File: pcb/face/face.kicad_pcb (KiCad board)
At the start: 2 copper layers, 130 x 65 mm, 27 parts, among them J1 26 pin IDC, J2 Phoenix MSTB, U1 K155ID1, U2 K155ID1, U3 K155ID1, U4 K155ID1

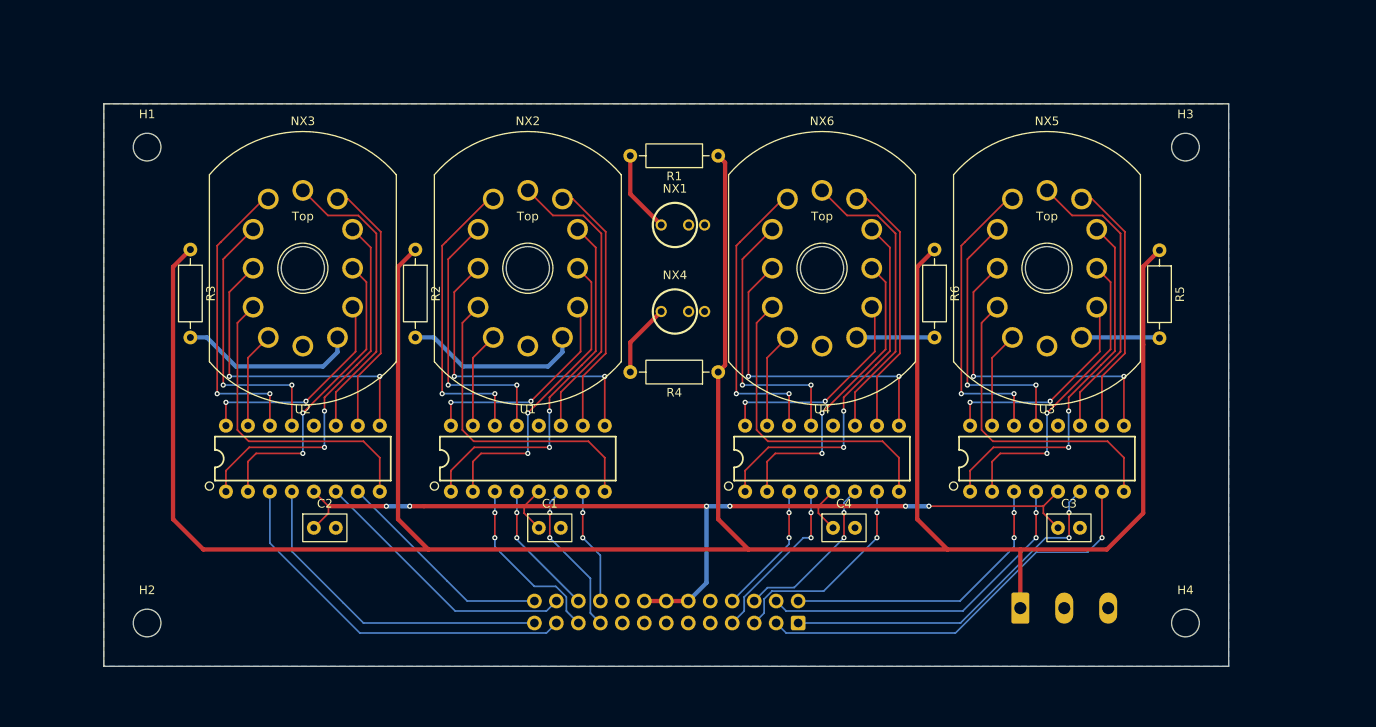
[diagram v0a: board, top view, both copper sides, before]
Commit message: Clock Face Rev C
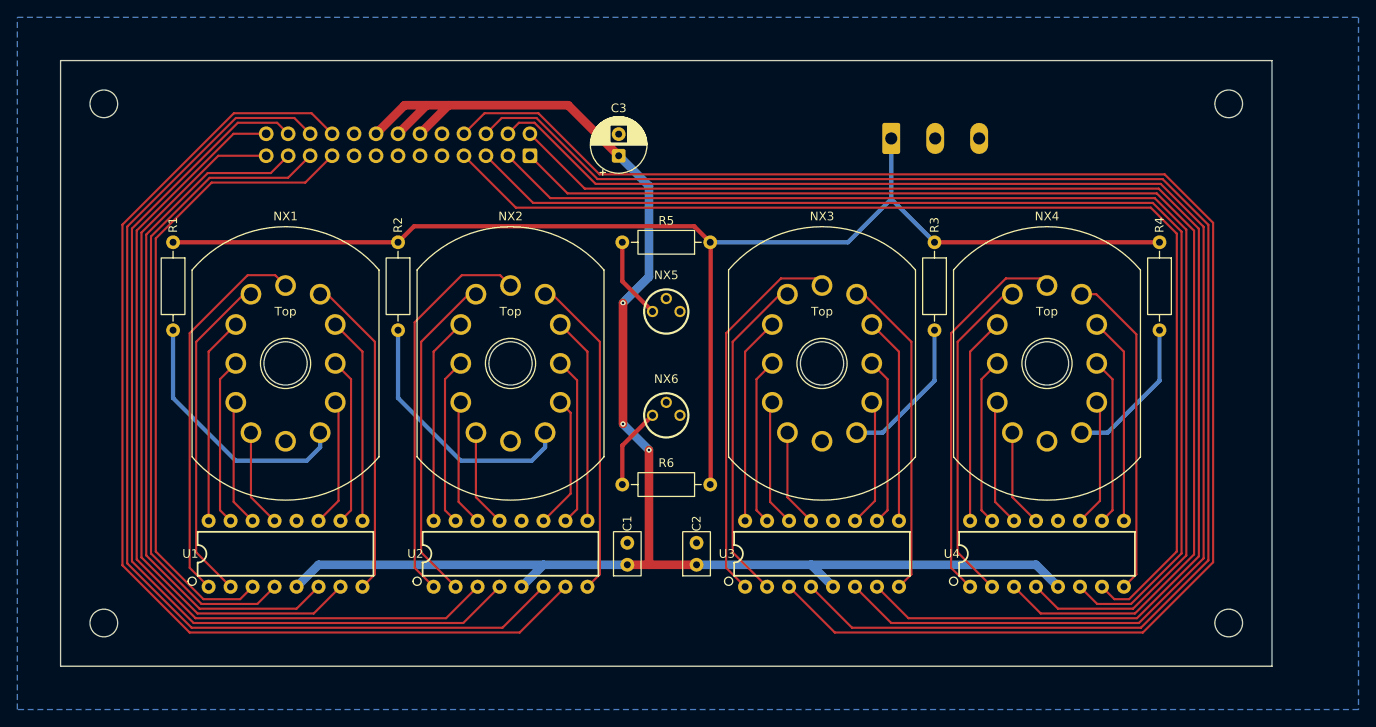
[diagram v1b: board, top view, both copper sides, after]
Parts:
- removed the C1 at (136.5, 109.0)
- C3: value 100nF -> 47uF; footprint 0_nixie_clock:C_Rect_L5.1mm_W3.2mm_P2.54mm_Goldmax -> 0_nixie_clock:CP_Radial_D6.3mm_P2.50mm
- moved C3 67.5 mm to (144.5, 66.0), turned to 90 degrees
- moved J1 62.3 mm to (134.2, 66.0)
- moved J2 56.3 mm to (176.0, 64.0)
- moved REF** 52.2 mm to (163.0, 64.0)
- moved C1 35.1 mm to (145.5, 112.0), turned to 90 degrees
- moved C2 17.3 mm to (153.5, 112.0), turned to 90 degrees
- moved R6 13.0 mm to (155.1, 104.0)
- moved NX6 12.0 mm to (150.0, 96.0)
- moved NX1 11.2 mm to (106.0, 90.0)
- moved NX2 11.2 mm to (132.0, 90.0)
- moved U1 11.2 mm to (106.0, 112.0)
- moved U2 11.2 mm to (132.0, 112.0)
- moved NX3 11.0 mm to (168.0, 90.0)
- moved NX4 11.0 mm to (194.0, 90.0)
- moved U3 11.0 mm to (168.0, 112.0)
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- renumbered C2 to C1, C4 to C2, NX3 to NX1, NX6 to NX3, NX5 to NX4, NX1 to NX5, NX4 to NX6, R3 to R1, R6 to R3, R5 to R4, R1 to R5, R4 to R6, U2 to U1, U1 to U2, U4 to U3, U3 to U4
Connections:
- J1 pad 1: M1_{B} -> M1_{A}
- J1 pad 19: H1_{B} -> H10_{A}
- J1 pad 2: M1_{A} -> M10_{C}
- J1 pad 21: H1_{A} -> H10_{D}
- J1 pad 22: H1_{D} -> H1_{B}
- J1 pad 23: H10_{A} -> H10_{B}
- J1 pad 24: H10_{B} -> H1_{D}
- J1 pad 25: H10_{D} -> H10_{C}
- J1 pad 26: H10_{C} -> H1_{A}
- J1 pad 3: M1_{C} -> M1_{D}
- J1 pad 4: M1_{D} -> M10_{B}
- J1 pad 5: M10_{C} -> M1_{B}
- J1 pad 6: M10_{B} -> M10_{D}
- J1 pad 7: M10_{D} -> M1_{C}
- NX1 pad 0: /NX1_{0} -> NX1_{0}
- NX1 pad 1: /NX1_{1} -> NX1_{1}
- NX1 pad 2: /NX1_{2} -> NX1_{2}
- NX1 pad 3: /NX1_{3} -> NX1_{3}
- NX1 pad 4: /NX1_{4} -> NX1_{4}
- NX1 pad 5: /NX1_{5} -> NX1_{5}
- NX1 pad 6: /NX1_{6} -> NX1_{6}
- NX1 pad 7: /NX1_{7} -> NX1_{7}
- NX1 pad 8: /NX1_{8} -> NX1_{8}
- NX1 pad 9: /NX1_{9} -> NX1_{9}
- NX2 pad 0: /NX2_{0} -> NX2_{0}
- NX2 pad 1: /NX2_{1} -> NX2_{1}
- NX2 pad 2: /NX2_{2} -> NX2_{2}
- NX2 pad 3: /NX2_{3} -> NX2_{3}
- NX2 pad 4: /NX2_{4} -> NX2_{4}
- NX2 pad 5: /NX2_{5} -> NX2_{5}
- NX2 pad 6: /NX2_{6} -> NX2_{6}
- NX2 pad 7: /NX2_{7} -> NX2_{7}
- NX2 pad 8: /NX2_{8} -> NX2_{8}
- NX2 pad 9: /NX2_{9} -> NX2_{9}
- NX3 pad 0: /NX3_{0} -> NX3_{0}
- NX3 pad 1: /NX3_{1} -> NX3_{1}
- NX3 pad 2: /NX3_{2} -> NX3_{2}
- NX3 pad 3: /NX3_{3} -> NX3_{3}
- NX3 pad 4: /NX3_{4} -> NX3_{4}
- NX3 pad 5: /NX3_{5} -> NX3_{5}
- NX3 pad 6: /NX3_{6} -> NX3_{6}
- NX3 pad 7: /NX3_{7} -> NX3_{7}
- NX3 pad 8: /NX3_{8} -> NX3_{8}
- NX3 pad 9: /NX3_{9} -> NX3_{9}
- NX4 pad 0: /NX4_{0} -> NX4_{0}
- NX4 pad 1: /NX4_{1} -> NX4_{1}
- NX4 pad 2: /NX4_{2} -> NX4_{2}
- NX4 pad 3: /NX4_{3} -> NX4_{3}
- NX4 pad 4: /NX4_{4} -> NX4_{4}
- NX4 pad 5: /NX4_{5} -> NX4_{5}
- NX4 pad 6: /NX4_{6} -> NX4_{6}
- NX4 pad 7: /NX4_{7} -> NX4_{7}
- NX4 pad 8: /NX4_{8} -> NX4_{8}
- NX4 pad 9: /NX4_{9} -> NX4_{9}
- U1 pad 1: /NX1_{8} -> NX1_{6}
- U1 pad 10: /NX1_{7} -> NX1_{9}
- U1 pad 11: /NX1_{6} -> NX1_{0}
- U1 pad 13: /NX1_{4} -> NX1_{1}
- U1 pad 14: /NX1_{5} -> NX1_{2}
- U1 pad 15: /NX1_{1} -> NX1_{3}
- U1 pad 16: /NX1_{0} -> NX1_{4}
- U1 pad 2: /NX1_{9} -> NX1_{5}
- U1 pad 8: /NX1_{2} -> NX1_{7}
- U1 pad 9: /NX1_{3} -> NX1_{8}
- U2 pad 1: /NX2_{8} -> NX2_{6}
- U2 pad 10: /NX2_{7} -> NX2_{9}
- U2 pad 11: /NX2_{6} -> NX2_{0}
- U2 pad 13: /NX2_{4} -> NX2_{1}
- U2 pad 14: /NX2_{5} -> NX2_{2}
- U2 pad 15: /NX2_{1} -> NX2_{3}
- U2 pad 16: /NX2_{0} -> NX2_{4}
- U2 pad 2: /NX2_{9} -> NX2_{5}
- U2 pad 8: /NX2_{2} -> NX2_{7}
- U2 pad 9: /NX2_{3} -> NX2_{8}
- U3 pad 1: /NX3_{8} -> NX3_{6}
- U3 pad 10: /NX3_{7} -> NX3_{9}
- U3 pad 11: /NX3_{6} -> NX3_{0}
- U3 pad 13: /NX3_{4} -> NX3_{1}
- U3 pad 14: /NX3_{5} -> NX3_{2}
- U3 pad 15: /NX3_{1} -> NX3_{3}
- U3 pad 16: /NX3_{0} -> NX3_{4}
- U3 pad 2: /NX3_{9} -> NX3_{5}
- U3 pad 8: /NX3_{2} -> NX3_{7}
- U3 pad 9: /NX3_{3} -> NX3_{8}
- U4 pad 1: /NX4_{8} -> NX4_{6}
- U4 pad 10: /NX4_{7} -> NX4_{9}
- U4 pad 11: /NX4_{6} -> NX4_{0}
- U4 pad 13: /NX4_{4} -> NX4_{1}
- U4 pad 14: /NX4_{5} -> NX4_{2}
- U4 pad 15: /NX4_{1} -> NX4_{3}
- U4 pad 16: /NX4_{0} -> NX4_{4}
- U4 pad 2: /NX4_{9} -> NX4_{5}
- U4 pad 8: /NX4_{2} -> NX4_{7}
- U4 pad 9: /NX4_{3} -> NX4_{8}
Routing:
- net M10_{A}: track 15.4 -> 186.6 mm, vias 2 -> 0
- net M10_{D}: track 19.5 -> 179.2 mm, vias 2 -> 0
- net +170V: track 306.7 -> 154.7 mm
- net M10_{B}: track 19.3 -> 169.3 mm, vias 2 -> 0
- net M10_{C}: track 24.6 -> 161.4 mm, vias 2 -> 0
- net H1_{C}: track 13.5 -> 126.5 mm, vias 2 -> 0
- net M1_{A}: track 33.9 -> 142.7 mm, vias 2 -> 0
- net M1_{D}: track 39.4 -> 140.6 mm, vias 2 -> 0
- net H1_{B}: track 18.1 -> 119.2 mm, vias 2 -> 0
- net M1_{B}: track 41.3 -> 136.2 mm, vias 2 -> 0
- net H1_{D}: track 15.6 -> 109.3 mm, vias 2 -> 0
- net M1_{C}: track 48.0 -> 134.4 mm, vias 1 -> 0
- net H1_{A}: track 20.6 -> 101.3 mm, vias 2 -> 0
- net +5V: track 121.9 -> 189.7 mm, vias 6 -> 3
- net H10_{C}: track 25.6 -> 82.6 mm
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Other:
- board size 130 x 65 mm -> 140 x 70 mm
